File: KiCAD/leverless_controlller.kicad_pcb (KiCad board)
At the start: 2 copper layers, 251.4 x 138.3 mm, 31 parts, among them SW2 SW_Push, U1 RP2040, U2 NCP1117-3.3_SOT223, U3 W25Q16JVSS, Y1 ABM8-272-T3

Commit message: Start PCB Layout
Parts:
- added J1: USB_C_Receptacle_USB2.0_14P, Fightstick_Library:USB_C_Receptacle_HCTL_Fightstick_16P_TopMnt_Horizontal, F.Cu at (76.4, 30.7)
- added SW10_SHARE1: SW_Push, Fightstick_Library:Kailh_MX_Style_Keyswitch, F.Cu at (257.2, 46.9)
- added SW11_START1: SW_Push, Fightstick_Library:Kailh_MX_Style_Keyswitch, F.Cu at (257.2, 63.1)
- added SW12_THROW1: SW_Push, Fightstick_Library:Kailh_MX_Style_Keyswitch, F.Cu at (149.9, 60.3)
- added SW13_R3: SW_Push, Fightstick_Library:Kailh_MX_Style_Keyswitch, F.Cu at (257.2, 95.4)
- added SW14_PS1: SW_Push, Fightstick_Library:Kailh_MX_Style_Keyswitch, F.Cu at (257.2, 111.5)
- added SW15_TOUCHPAD1: SW_Push, Fightstick_Library:Kailh_MX_Style_Keyswitch, F.Cu at (257.2, 127.7)
- added SW16_UP1: SW_Push, Fightstick_Library:Kailh_MX_Style_Keyswitch, F.Cu at (150.4, 136.0)
- added SW17_UP2: SW_Push, Fightstick_Library:Kailh_MX_Style_Keyswitch, F.Cu at (117.1, 54.4)
- added SW18_DOWN1: SW_Push, Fightstick_Library:Kailh_MX_Style_Keyswitch, F.Cu at (109.8, 72.0)
- added SW19_LEFT1: SW_Push, Fightstick_Library:Kailh_MX_Style_Keyswitch, F.Cu at (92.2, 64.7)
- added SW20_RIGHT1: SW_Push, Fightstick_Library:Kailh_MX_Style_Keyswitch, F.Cu at (125.9, 83.0)
- added SW3_MK1: SW_Push, Fightstick_Library:Kailh_MX_Style_Keyswitch, F.Cu at (199.9, 90.0)
- added SW4_LP1: SW_Push, Fightstick_Library:Kailh_MX_Style_Keyswitch, F.Cu at (174.9, 75.0)
- added SW5_MP1: SW_Push, Fightstick_Library:Kailh_MX_Style_Keyswitch, F.Cu at (199.9, 61.0)
- added SW6_DI1: SW_Push, Fightstick_Library:Kailh_MX_Style_Keyswitch, F.Cu at (175.1, 46.0)
- added SW7_HP1: SW_Push, Fightstick_Library:Kailh_MX_Style_Keyswitch, F.Cu at (228.9, 61.0)
- added SW8_DP1: SW_Push, Fightstick_Library:Kailh_MX_Style_Keyswitch, F.Cu at (60.0, 72.0)
- added SW9_HK1: SW_Push, Fightstick_Library:Kailh_MX_Style_Keyswitch, F.Cu at (228.9, 90.0)
- S1: footprint keyswitches.pretty-2.1:Stabilizer_MX_2u -> Fightstick_Library:Kailh_MX_Style_Keyswitch
- SW2_LK1: renamed from SW2; footprint keyswitches.pretty-2.1:Kailh_socket_MX -> Fightstick_Library:Kailh_MX_Style_Keyswitch
- moved C2 100.1 mm to (59.9, 40.6), turned to 180 degrees
- moved C1 94.0 mm to (68.9, 35.7), turned to 180 degrees
- moved R1 92.3 mm to (69.5, 33.7), turned to 180 degrees
- moved U2 90.5 mm to (65.9, 40.7), turned to 180 degrees
- moved C5 89.7 mm to (72.9, 45.5), turned to 180 degrees
- moved R2 87.8 mm to (73.9, 37.2), turned to -90 degrees
- moved R6 87.6 mm to (70.6, 50.4), turned to -90 degrees
- moved R5 87.1 mm to (68.3, 53.1)
- moved R3 86.1 mm to (78.4, 36.3)
- moved SW2_LK1 75.7 mm to (174.9, 104.0)
- moved C4 74.8 mm to (95.9, 39.4), turned to 180 degrees
- moved R4 73.4 mm to (91.4, 42.9), turned to 180 degrees
- moved C17 68.6 mm to (83.6, 36.3), turned to 90 degrees
- moved C3 68.5 mm to (99.0, 43.2), turned to -90 degrees
- moved C16 67.2 mm to (82.5, 36.3), turned to 90 degrees
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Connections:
- SW2_LK1 pad 1: A1 -> B1
- U1 pad 34: unconnected-(U1-GPIO22-Pad34) -> UP2
- U1 pad 4: UP -> UP1
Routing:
- net +3.3V: track 0.00 -> 66.5 mm
- net /Main/QSPI_SS: track 0.00 -> 28.9 mm
- net +1V1: track 0.00 -> 18.2 mm
- net /Main/QSPI_SD1: track 0.00 -> 15.2 mm
- net /Main/XIN: track 0.00 -> 12.4 mm
- net /Main/QSPI_SD2: track 0.00 -> 11.9 mm
- net VBUS: track 0.00 -> 10.8 mm
- net /Main/D+: track 0.00 -> 10.6 mm
- net /Main/D-: track 0.00 -> 8.32 mm
- net /Main/QSPI_SD3: track 0.00 -> 6.70 mm
- net /Main/QSPI_SCLK: track 0.00 -> 6.15 mm
- net Net-(C4-Pad2): track 0.00 -> 6.10 mm
- net /Main/QSPI_SD0: track 0.00 -> 4.63 mm
- net /Main/XOUT: track 0.00 -> 3.02 mm
- net Net-(U1-USB_DP): track 0.00 -> 2.55 mm
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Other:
- board outline removed

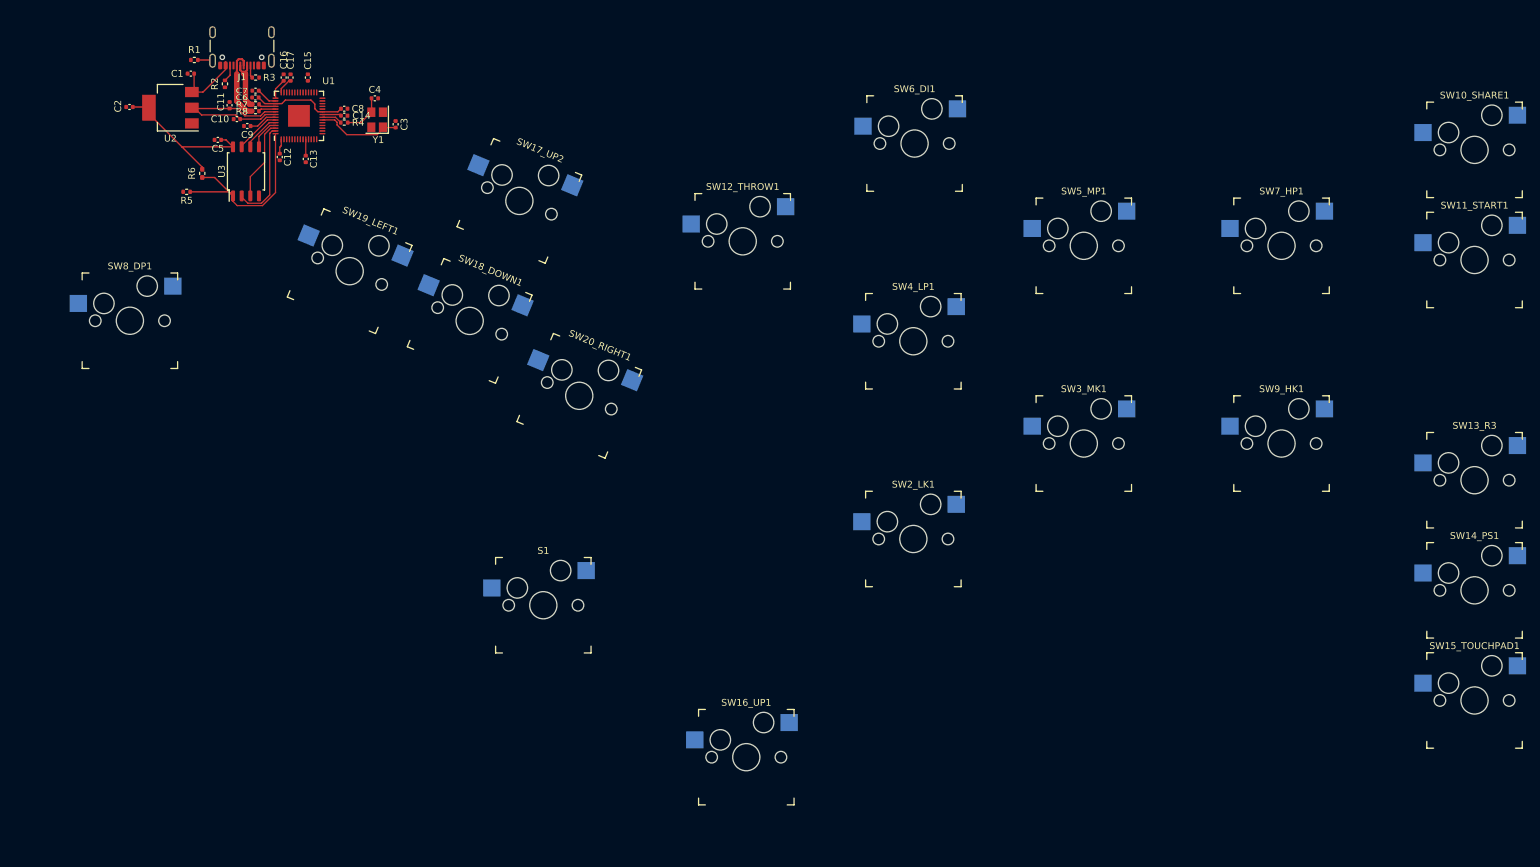
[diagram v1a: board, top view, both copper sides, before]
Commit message: PCB First Draft
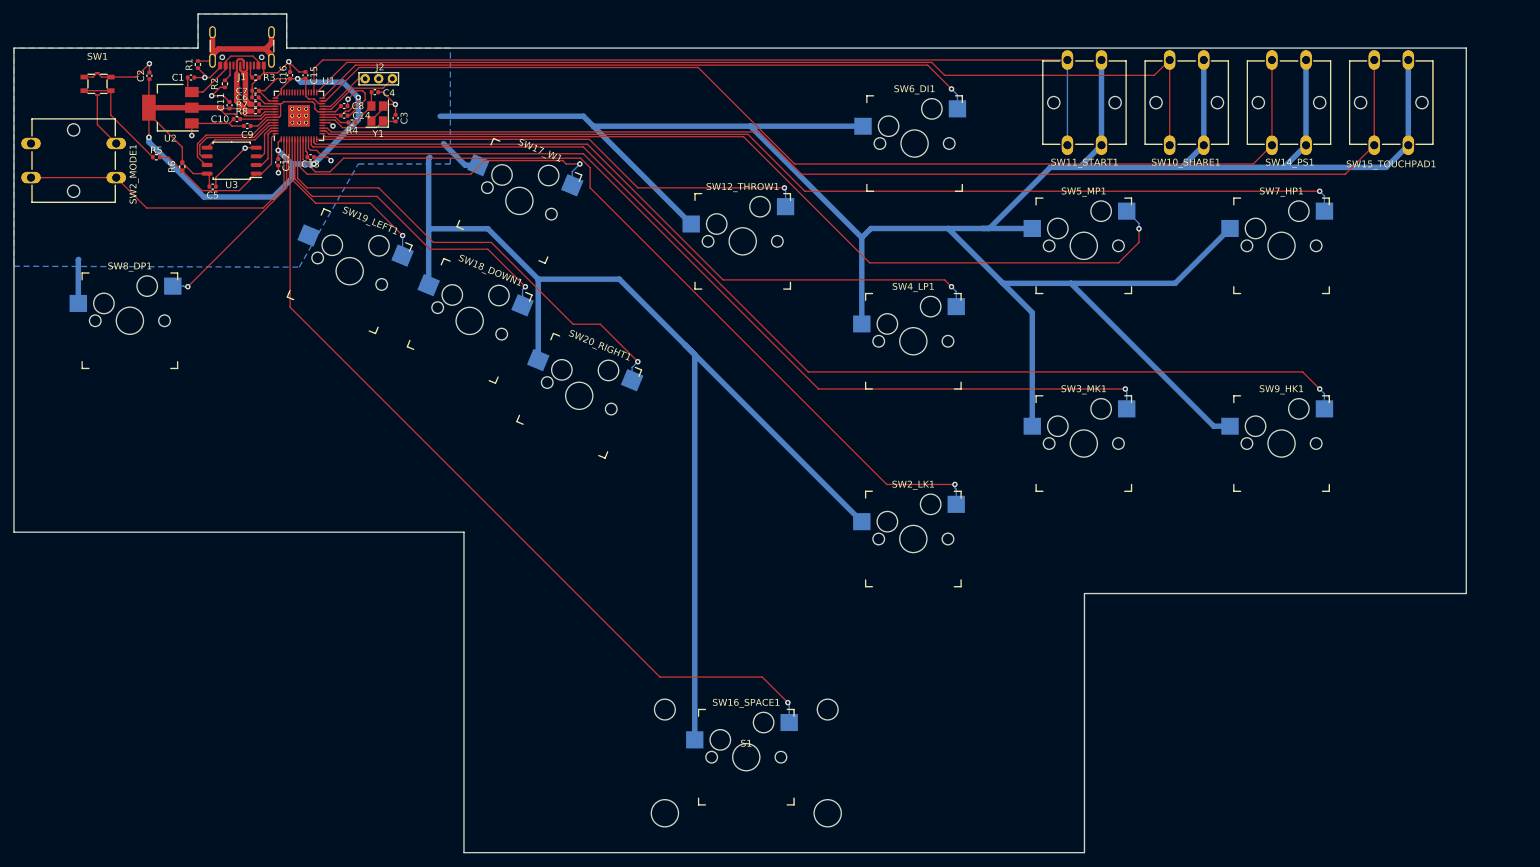
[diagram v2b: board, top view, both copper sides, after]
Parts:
- removed C17: 100n, Capacitor_SMD:C_0402_1005Metric
- removed SW13_R3: SW_Push, Fightstick_Library:Kailh_MX_Style_Keyswitch
- added ?: , , F.Cu at (83.8, 41.9)
- added ?: , , F.Cu at (85.9, 41.9)
- added ?: , , F.Cu at (85.9, 40.9)
- added ?: , , F.Cu at (85.9, 42.9)
- added ?: , , F.Cu at (84.8, 42.9)
- added ?: , , F.Cu at (84.8, 40.9)
- added ?: , , F.Cu at (84.8, 41.9)
- added ?: , , F.Cu at (83.8, 42.9)
- added ?: , , F.Cu at (83.8, 40.9)
- added J2: Conn_01x03_Socket, Fightstick_Library:Debug_Points, F.Cu at (97.8, 36.5)
- added SW1: SW_DIP_x01, Fightstick_Library:SW_SMD_BUTTON_YTS_A007, F.Cu at (55.2, 37.2)
- added SW2_MODE1: SW_SPST, Button_Switch_THT:SW_SPST_Omron_B3F-40xx, F.Cu at (58.0, 51.0)
- S1: footprint Fightstick_Library:Kailh_MX_Style_Keyswitch -> PCM_Mounting_Keyboard_Stabilizer:Stabilizer_Cherry_MX_2.00u
- SW10_SHARE1, SW11_START1, SW14_PS1, SW15_TOUCHPAD1: footprint Fightstick_Library:Kailh_MX_Style_Keyswitch -> Button_Switch_THT:SW_SPST_Omron_B3F-40xx
- moved SW15_TOUCHPAD1 82.7 mm to (242.5, 46.2), turned to 90 degrees
- moved SW14_PS1 71.7 mm to (227.5, 46.2), turned to 90 degrees
- moved SW11_START1 62.0 mm to (197.5, 46.2), turned to 90 degrees
- moved SW10_SHARE1 44.7 mm to (212.5, 46.2), turned to 90 degrees
- moved S1 37.2 mm to (150.4, 136.0)
- moved C5 6.90 mm to (72.1, 52.3), turned to 0 degrees
- moved R5 6.75 mm to (63.9, 48.0)
- moved C2 5.43 mm to (62.9, 36.1), turned to 90 degrees
- moved R6 3.08 mm to (67.7, 49.4)
- moved U3 2.62 mm to (74.9, 48.5), turned to 180 degrees
- moved R4 1.14 mm to (92.6, 42.9)
- moved C16 1.00 mm to (83.5, 36.0)
- moved C3 0.90 mm to (99.0, 42.3)
- moved Y1 0.90 mm to (96.3, 41.6)
- moved C4 0.90 mm to (95.9, 38.5)
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- renumbered SW16_UP1 to SW16_SPACE1, SW17_UP2 to SW17_W1
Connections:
- net UP1 renamed SPACE
- SW17_W1 pad 1: UP2 -> W
- U1 pad 11: R2 -> B2
- U1 pad 12: L2 -> R2
- U1 pad 14: B4 -> L3
- U1 pad 15: R1 -> B4
- U1 pad 16: L1 -> R1
- U1 pad 17: TURBO -> A2
- U1 pad 18: T LED -> unconnected-(U1-GPIO15-Pad18)
- U1 pad 2: SDA -> MODE
- U1 pad 26: /Main/RUN -> +3.3V
- U1 pad 27: S1 -> A1
- U1 pad 28: S2 -> L1
- U1 pad 29: L3 -> S1
- U1 pad 3: SLC -> L2
- U1 pad 30: R3 -> S2
- U1 pad 31: A1 -> unconnected-(U1-GPIO20-Pad31)
- U1 pad 32: A2 -> unconnected-(U1-GPIO21-Pad32)
- U1 pad 34: UP2 -> unconnected-(U1-GPIO22-Pad34)
- U1 pad 5: DOWN -> LEFT
- U1 pad 6: RIGHT -> DOWN
- U1 pad 7: LEFT -> RIGHT
- U1 pad 8: B1 -> W
- U1 pad 9: B2 -> B1
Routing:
- net GND: track 0.00 -> 654.5 mm, vias 0 -> 11
- net A2: track 0.00 -> 171.3 mm
- net R2: track 0.00 -> 166.8 mm, vias 0 -> 1
- net A1: track 0.00 -> 160.8 mm
- net R1: track 0.00 -> 153.1 mm, vias 0 -> 1
- net S1: track 0.00 -> 141.1 mm
- net B2: track 0.00 -> 138.7 mm, vias 0 -> 1
- net B4: track 0.00 -> 134.2 mm, vias 0 -> 1
- net S2: track 0.00 -> 127.0 mm
- net B1: track 0.00 -> 124.7 mm, vias 0 -> 1
- net SPACE: track 0.00 -> 124.7 mm, vias 0 -> 1
- net B3: track 0.00 -> 106.0 mm, vias 0 -> 1
- net L1: track 0.00 -> 99.0 mm, vias 0 -> 1
- net +3.3V: track 66.5 -> 144.8 mm, vias 0 -> 5
- net L3: track 0.00 -> 74.4 mm, vias 0 -> 1
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- added copper zone on B.Cu, net GND
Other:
- board outline added: 213 x 123 mm
